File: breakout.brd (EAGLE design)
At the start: 25.4 x 32.4 mm, 26 parts, among them IC2 REG1117, Q1 12Mhz, U1 LM358DR

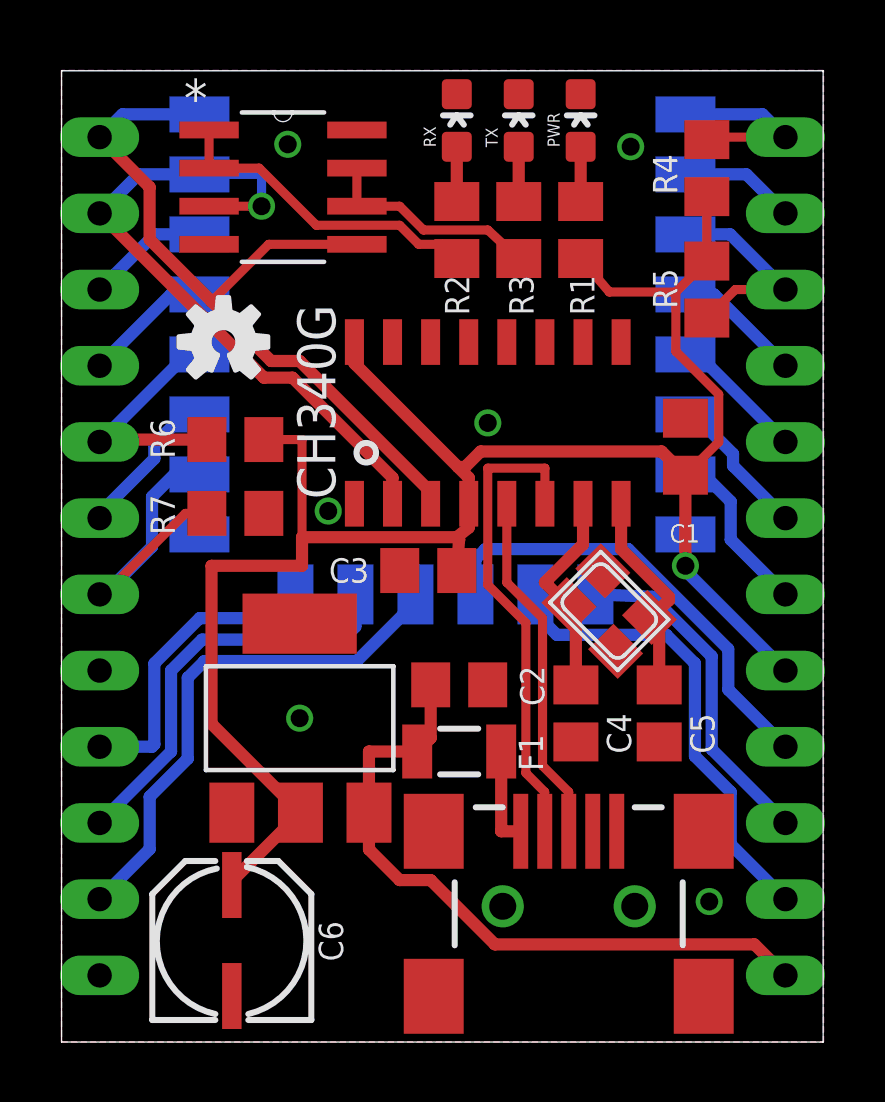
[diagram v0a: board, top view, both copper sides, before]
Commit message: adding some dimentions
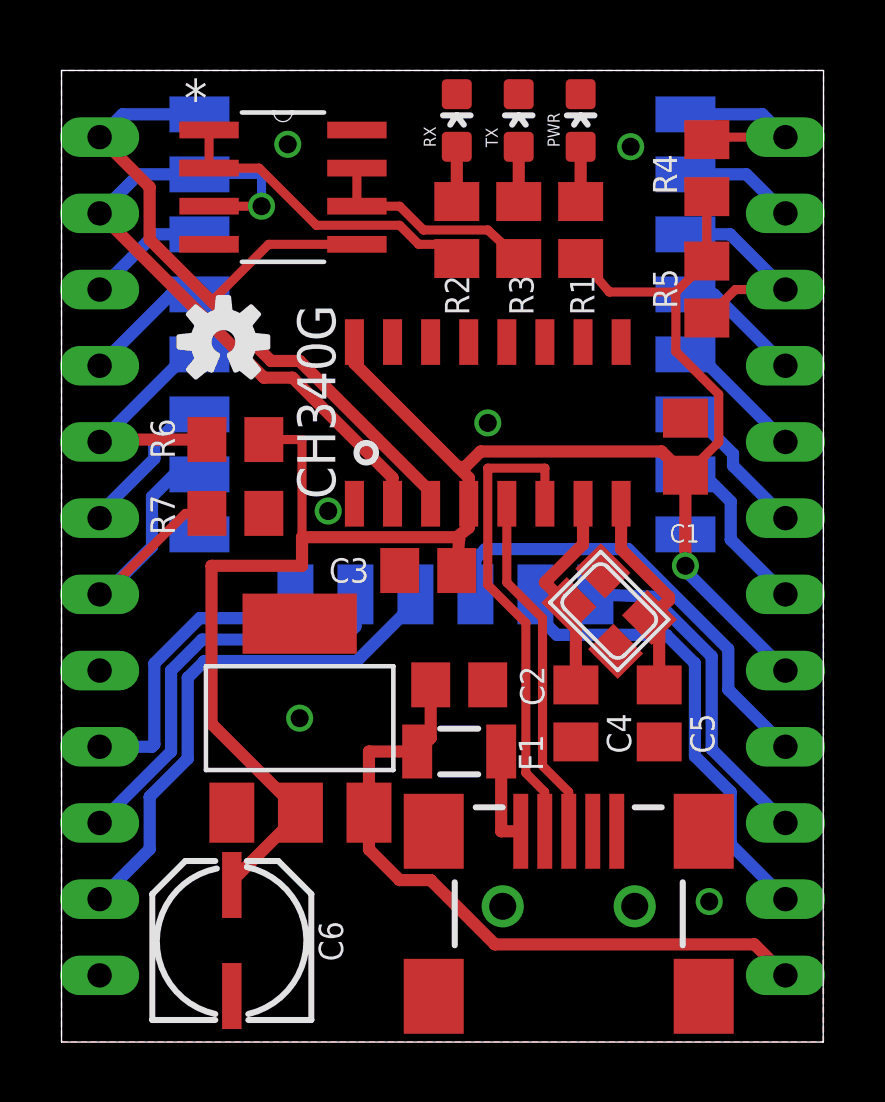
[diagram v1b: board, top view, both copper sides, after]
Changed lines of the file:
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@@
 <grid distance="0.003125" unitdist="inch" unit="inch" style="lines" multiple="1" display="no" altdistance="0.025" altunitdist="inch" altunit="inch"/>
 <layers>
-<layer number="1" name="Top" color="4" fill="1" visible="no" active="yes"/>
+<layer number="1" name="Top" color="4" fill="1" visible="yes" active="yes"/>
 <layer number="2" name="Route2" color="1" fill="3" visible="yes" active="yes"/>
 <layer number="3" name="Route3" color="4" fill="3" visible="no" active="yes"/>
@@
 <plain>
 <wire x1="0" y1="0" x2="25.3875" y2="0" width="0" layer="20"/>
-<wire x1="25.3875" y1="0" x2="25.3875" y2="32.375" width="0" layer="20"/>
-<wire x1="25.3875" y1="32.375" x2="0" y2="32.375" width="0" layer="20"/>
-<wire x1="0" y1="32.375" x2="0" y2="0" width="0" layer="20"/>
+<wire x1="25.3875" y1="0" x2="25.4" y2="32.385" width="0" layer="20"/>
+<wire x1="25.4" y1="32.385" x2="0" y2="32.385" width="0" layer="20"/>
+<wire x1="0" y1="32.385" x2="0" y2="0" width="0" layer="20"/>
 <text x="22.304375" y="9.2075" size="1.4224" layer="26" rot="MR0">git.io/vwtq7</text>
 <text x="22.304375" y="6.82625" size="1.4224" layer="26" rot="MR0">@matthewbaggett</text>
+<dimension x1="1.27" y1="30.1625" x2="24.13" y2="30.1625" x3="12.7" y3="38.25875" textsize="5.08" layer="150"/>
+<dimension x1="0" y1="0" x2="25.4" y2="0" x3="12.7" y3="-11.509375" textsize="5.08" layer="150"/>
+<dimension x1="25.3875" y1="0" x2="25.4" y2="32.385" x3="34.443565625" y3="16.18900625" textsize="5.08" layer="150"/>
+<dimension x1="1.27" y1="30.1625" x2="1.27" y2="27.6225" x3="-5.08" y3="28.8925" textsize="5.08" layer="150"/>
+<dimension x1="17.859375" y1="39.0525" x2="17.859375" y2="-1.42875" x3="46.273321875" y3="18.811875" textsize="5.08" layer="150"/>
 </plain>
 <attributes>
